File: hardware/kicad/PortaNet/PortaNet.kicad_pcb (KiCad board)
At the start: 2 copper layers, 23 parts, among them J1 SMA, J2 Molex 0480370001, J4 RST, U1 ESP32-C3, U2 AP2114HA-3.3TRG1, Y1 FL400WFQA1

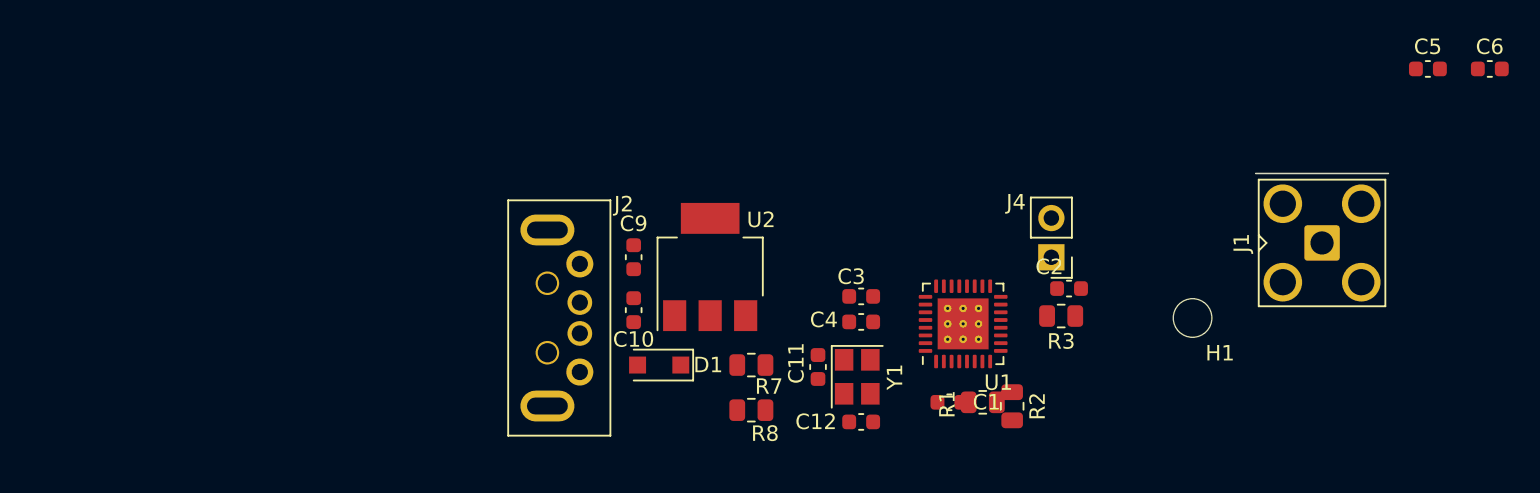
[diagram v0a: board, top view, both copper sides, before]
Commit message: v4
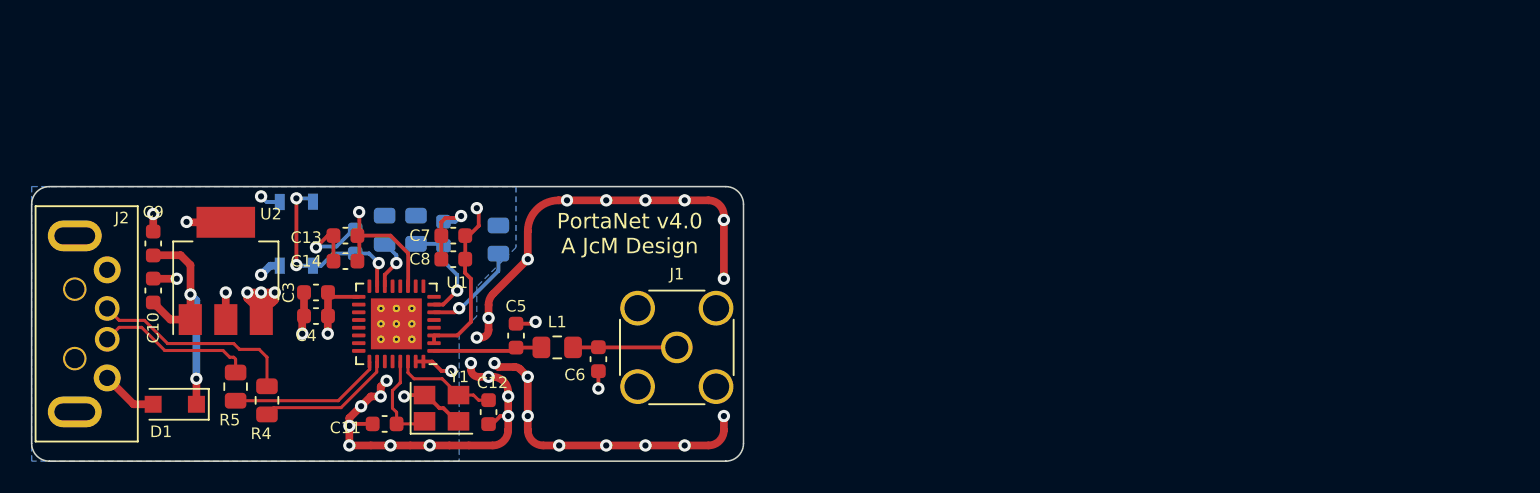
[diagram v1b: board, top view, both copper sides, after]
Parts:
- removed H1: MountingHole, MountingHole:MountingHole_2.5mm
- removed J4: RST, Connector_PinHeader_2.54mm:PinHeader_1x02_P2.54mm_Vertical
- removed R7, R8: 22, Resistor_SMD:R_0805_2012Metric
- added C13: 0.1uF, Capacitor_SMD:C_0603_1608Metric, F.Cu at (111.4, 65.8)
- added C14: 10uF, Capacitor_SMD:C_0603_1608Metric, F.Cu at (111.4, 67.4)
- added C7: 0.1uF, Capacitor_SMD:C_0603_1608Metric, F.Cu at (118.4, 65.8)
- added C8: 10uF, Capacitor_SMD:C_0603_1608Metric, F.Cu at (118.4, 67.3)
- added L1: TBD, Inductor_SMD:L_0805_2012Metric_Pad1.15x1.40mm_HandSolder, F.Cu at (125.1, 73.0)
- added R4: 22, Resistor_SMD:R_0805_2012Metric, F.Cu at (106.3, 76.5)
- added R5: 22, Resistor_SMD:R_0805_2012Metric, F.Cu at (104.3, 75.6)
- added SW1: 434133025816, Button_Switch_SMD:SW_Push_1P1T_NO_Vertical_Wuerth_434133025816, B.Cu at (108.2, 65.7)
- C1, C2, R1, R2, R3: moved to B.Cu
- J1: footprint Connector_Coaxial:SMA_Amphenol_901-143_Horizontal -> Connector_Coaxial:SMA_Amphenol_132134_Vertical
- moved C5 61.5 mm to (122.4, 72.3), turned to 90 degrees
- moved C6 60.7 mm to (127.8, 73.8), turned to -90 degrees
- moved C2 46.3 mm to (112.0, 66.2), turned to 90 degrees
- moved R3 44.2 mm to (113.9, 65.4), turned to 90 degrees
- moved J1 42.3 mm to (132.8, 73.0)
- moved R1 38.4 mm to (116.0, 65.4), turned to 90 degrees
- moved U1 36.7 mm to (114.7, 71.5), turned to 180 degrees
- moved C4 35.3 mm to (109.5, 71.0)
- moved C3 35.3 mm to (109.5, 69.5)
- moved R2 35.0 mm to (121.3, 66.0), turned to 90 degrees
- moved C1 34.5 mm to (117.7, 65.7), turned to 90 degrees
- moved D1 31.5 mm to (100.3, 76.7)
- moved U2 31.4 mm to (103.6, 68.1)
- moved C10 31.1 mm to (98.9, 69.3), turned to 90 degrees
- moved C9 31.1 mm to (98.9, 66.3)
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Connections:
- J2 pad 2: Net-(J2-Pad2) -> /misc1/D-
- J2 pad 3: Net-(J2-Pad3) -> /misc1/D+
- J2 pad 5: GND -> unconnected-(J2-Pad5)
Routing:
- net GND: track 0.00 -> 103.3 mm, vias 0 -> 40
- net 3V3: track 0.00 -> 35.3 mm, vias 0 -> 7
- net 5V: track 0.00 -> 16.3 mm, vias 0 -> 2
- net /misc1/D+: track 0.00 -> 13.5 mm
- net Net-(C2-Pad1): track 0.00 -> 13.0 mm, vias 0 -> 3
- net /misc1/D-: track 0.00 -> 10.4 mm
- net USB_DN: track 0.00 -> 10.0 mm
- net USB_DP: track 0.00 -> 8.94 mm
- net ANT: track 0.00 -> 7.05 mm
- net Net-(C1-Pad1): track 0.00 -> 6.98 mm, vias 0 -> 1
- net Net-(C6-Pad1): track 0.00 -> 6.73 mm
- net XTAL_P: track 0.00 -> 6.68 mm
- net XTAL_N: track 0.00 -> 6.44 mm
- net Net-(U1-Pad6): track 0.00 -> 6.40 mm, vias 0 -> 1
- net Net-(D1-Pad2): track 0.00 -> 3.68 mm
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- added copper zone on B.Cu, net 3V3
- added copper zone on In1.Cu, net GND
- added copper zone on In2.Cu, net GND
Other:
- board outline added: 46.1 x 17.8 mm
- copper layers 2 -> 4
- board text added: "LAYER 1"
- board text added: "LAYERING"
- board text added: "PWR/Signals"
- board text added: "PWR/USB"
- board text added: "PortaNet v4.0 A JcM Design"
- board text added: "RF"
- board text added: "Signals"
- board text added: "XTAL"
- board text added: "uC"
- board text removed: "3.3V"
- board text removed: "5V"
- board text removed: "PortaNet v4.0, A JCM Design"
- board text removed: "RX"
- board text removed: "TX"
